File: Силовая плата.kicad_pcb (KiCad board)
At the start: 6 copper layers, 67 x 90.5 mm, 71 parts, among them J1 A, J2 A, J3 B, J4 C, J5 IN-, J6 IN+, J7 Conn_02x10_Odd_Even, J8 A, Q1 2N7002, Q2 2N7002, Q3 2N7002, Q4 2N7002, Q5 2N7002, Q6 2N7002, Q7 BSS214NW

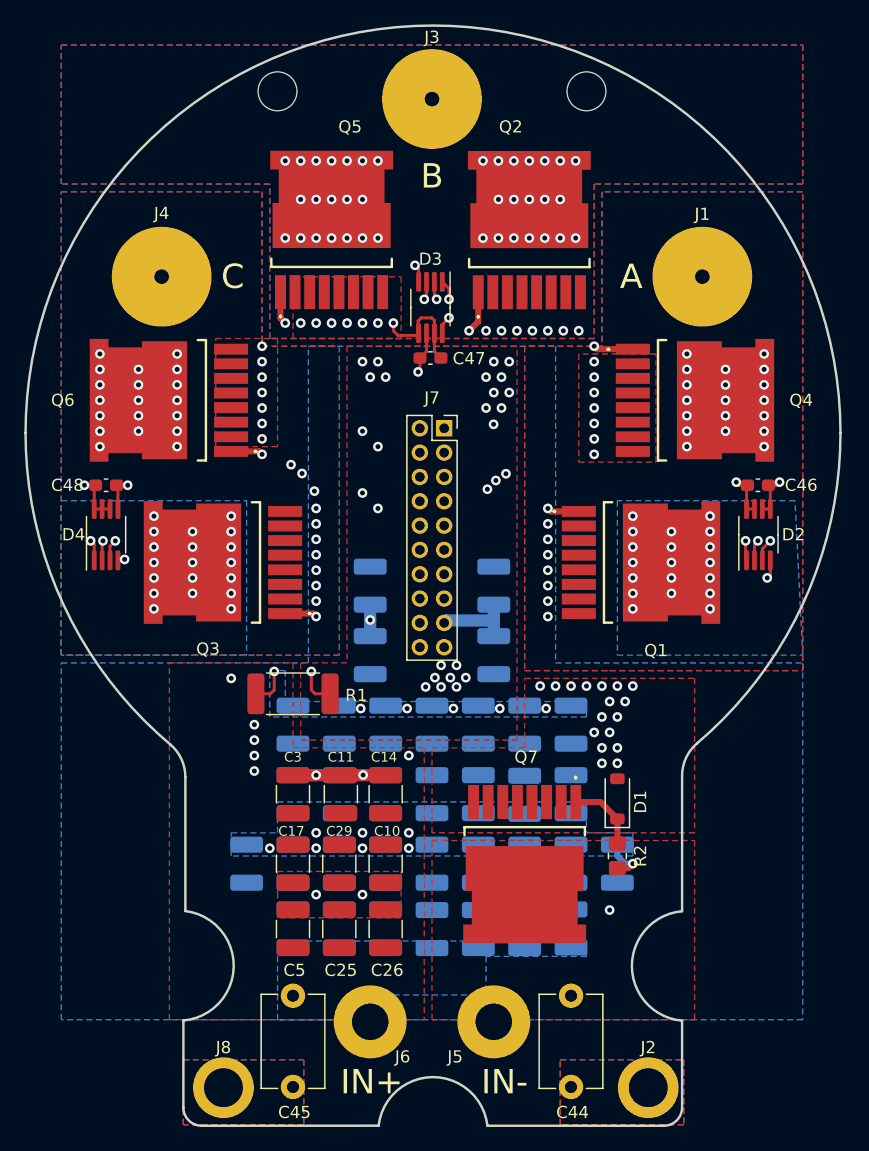
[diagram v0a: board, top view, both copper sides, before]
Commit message: Первый вариант
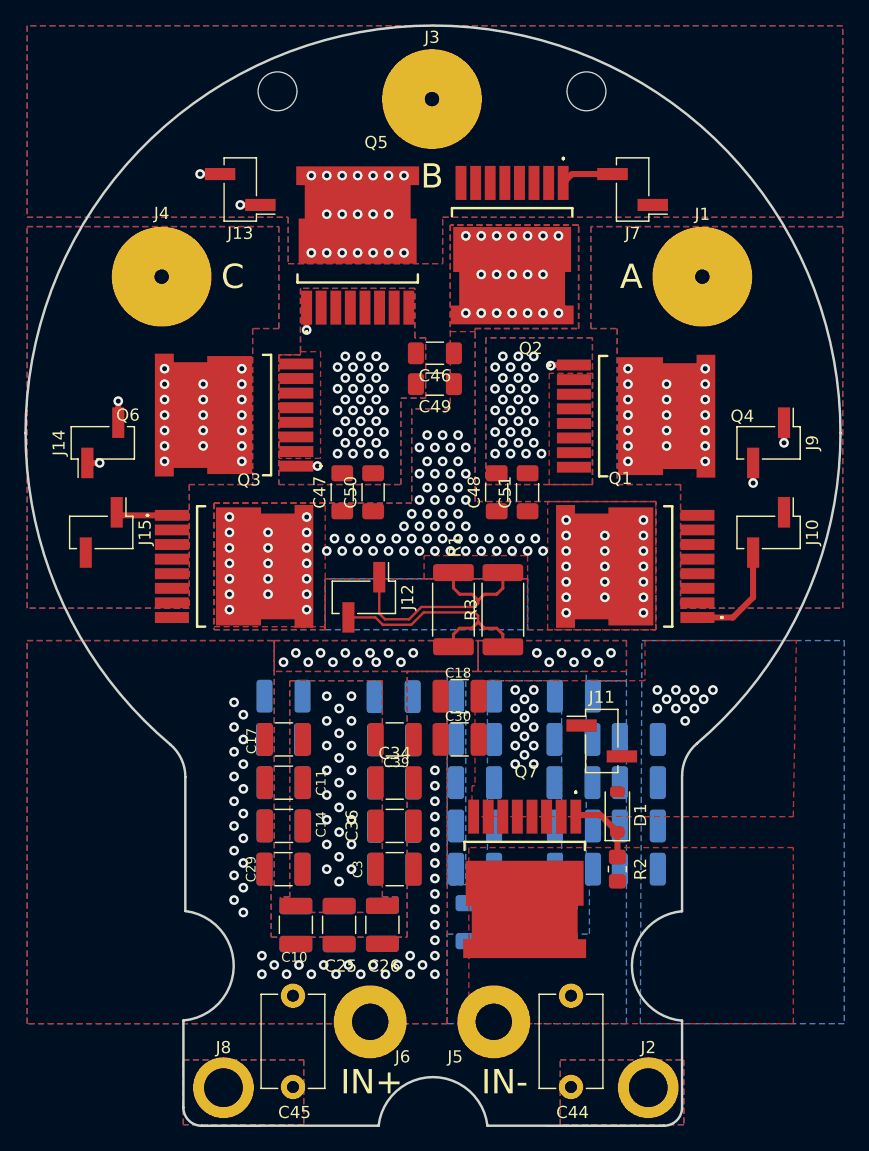
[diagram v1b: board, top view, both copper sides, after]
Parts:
- removed D2, D3, D4: STLM75DS2F, Package_SO:MSOP-8_3x3mm_P0.65mm
- added C49: 10u, Capacitor_SMD:C_1206_3216Metric_Pad1.33x1.80mm_HandSolder, F.Cu at (149.6, 67.1)
- added C50: 10u, Capacitor_SMD:C_1206_3216Metric_Pad1.33x1.80mm_HandSolder, F.Cu at (144.5, 75.9)
- added C51: 10u, Capacitor_SMD:C_1206_3216Metric_Pad1.33x1.80mm_HandSolder, F.Cu at (157.2, 75.9)
- added J10: Conn_01x02_Pin, Connector_PinHeader_2.54mm:PinHeader_1x02_P2.54mm_Vertical_SMD_Pin1Left, F.Cu at (177.0, 79.2)
- added J11: Conn_01x02_Pin, Connector_PinHeader_2.54mm:PinHeader_1x02_P2.54mm_Vertical_SMD_Pin1Left, F.Cu at (163.3, 96.4)
- added J12: Conn_01x02_Pin, Connector_PinHeader_2.54mm:PinHeader_1x02_P2.54mm_Vertical_SMD_Pin1Left, F.Cu at (143.8, 84.6)
- added J13: Conn_01x02_Pin, Connector_PinHeader_2.54mm:PinHeader_1x02_P2.54mm_Vertical_SMD_Pin1Left, F.Cu at (133.6, 51.1)
- added J14: Conn_01x02_Pin, Connector_PinHeader_2.54mm:PinHeader_1x02_P2.54mm_Vertical_SMD_Pin1Left, F.Cu at (122.3, 71.9)
- added J15: Conn_01x02_Pin, Connector_PinHeader_2.54mm:PinHeader_1x02_P2.54mm_Vertical_SMD_Pin1Left, F.Cu at (122.2, 79.2)
- added J9: Conn_01x02_Pin, Connector_PinHeader_2.54mm:PinHeader_1x02_P2.54mm_Vertical_SMD_Pin1Left, F.Cu at (177.0, 71.9)
- added R3: PU2512FKGP60U5L, Resistor_SMD:R_2512_6332Metric_Pad1.40x3.35mm_HandSolder, F.Cu at (155.2, 85.6)
- C18, C30, C34, C36, C39: moved to F.Cu
- C46, C47, C48: value 0.1u -> 10u; footprint Capacitor_SMD:C_0603_1608Metric_Pad1.08x0.95mm_HandSolder -> Capacitor_SMD:C_1206_3216Metric_Pad1.33x1.80mm_HandSolder
- C5: moved to B.Cu
- J7: value Conn_02x10_Odd_Even -> Conn_01x02_Pin; footprint Connector_PinSocket_2.00mm:PinSocket_2x10_P2.00mm_Vertical -> Connector_PinHeader_2.54mm:PinHeader_1x02_P2.54mm_Vertical_SMD_Pin1Left
- moved C12 32.4 mm to (166.4, 103.4), turned to 0 degrees
- moved C48 32.1 mm to (154.7, 75.9), turned to 90 degrees
- moved C5 30.0 mm to (161.0, 92.7), turned to 180 degrees
- moved C22 28.8 mm to (166.4, 99.8), turned to 0 degrees
- moved C46 28.7 mm to (149.6, 64.5), turned to 180 degrees
- moved C24 28.4 mm to (166.4, 106.9), turned to 0 degrees
- moved C32 27.4 mm to (137.2, 92.7), turned to 0 degrees
- moved J7 25.0 mm to (165.9, 51.1), turned to 180 degrees
- moved C28 24.5 mm to (160.0, 111.3)
- moved C23 24.1 mm to (137.1, 96.3), turned to 0 degrees
- moved C36 21.4 mm to (146.3, 103.4), turned to 180 degrees
- moved C39 21.0 mm to (146.3, 96.3), turned to 180 degrees
- moved C40 20.5 mm to (152.9, 92.7), turned to 0 degrees
- moved C16 20.3 mm to (161.0, 106.9), turned to 180 degrees
- moved C38 19.9 mm to (146.3, 103.4), turned to 180 degrees
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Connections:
- C1 pad 1: Shunt_1 -> Shunt+
- C10 pad 1: Shunt_1 -> Shunt+
- C11 pad 1: Shunt_1 -> Shunt+
- C12 pad 1: Shunt_1 -> Shunt+
- C13 pad 1: Shunt_1 -> Shunt+
- C14 pad 1: Shunt_1 -> Shunt+
- C15 pad 1: Shunt_1 -> Shunt+
- C16 pad 1: Shunt_1 -> Shunt+
- C17 pad 1: Shunt_1 -> Shunt+
- C18 pad 1: Shunt_1 -> Shunt+
- C19 pad 1: Shunt_1 -> Shunt+
- C2 pad 1: Shunt_1 -> Shunt+
- C20 pad 1: Shunt_1 -> Shunt+
- C21 pad 1: Shunt_1 -> Shunt+
- C22 pad 1: Shunt_1 -> Shunt+
- C23 pad 1: Shunt_1 -> Shunt+
- C24 pad 1: Shunt_1 -> Shunt+
- C25 pad 1: Shunt_1 -> Shunt+
- C26 pad 1: Shunt_1 -> Shunt+
- C27 pad 1: Shunt_1 -> Shunt+
- C28 pad 1: Shunt_1 -> Shunt+
- C29 pad 1: Shunt_1 -> Shunt+
- C3 pad 1: Shunt_1 -> Shunt+
- C30 pad 1: Shunt_1 -> Shunt+
- C31 pad 1: Shunt_1 -> Shunt+
- C32 pad 1: Shunt_1 -> Shunt+
- C33 pad 1: Shunt_1 -> Shunt+
- C34 pad 1: Shunt_1 -> Shunt+
- C35 pad 1: Shunt_1 -> Shunt+
- C36 pad 1: Shunt_1 -> Shunt+
- C37 pad 1: Shunt_1 -> Shunt+
- C38 pad 1: Shunt_1 -> Shunt+
- C39 pad 1: Shunt_1 -> Shunt+
- C4 pad 1: Shunt_1 -> Shunt+
- C40 pad 1: Shunt_1 -> Shunt+
- C41 pad 1: Shunt_1 -> Shunt+
- C42 pad 1: Shunt_1 -> Shunt+
- C43 pad 1: Shunt_1 -> Shunt+
- C45 pad 1: Shunt_1 -> Shunt+
- C46 pad 1: +3.3V -> Shunt-
- C47 pad 1: +3.3V -> Shunt-
- C48 pad 1: +3.3V -> Shunt-
- C5 pad 1: Shunt_1 -> Shunt+
- C6 pad 1: Shunt_1 -> Shunt+
- C7 pad 1: Shunt_1 -> Shunt+
- C8 pad 1: Shunt_1 -> Shunt+
- C9 pad 1: Shunt_1 -> Shunt+
- J6 pad 1: Shunt_1 -> Shunt+
- J7 pad 1: +3.3V -> B
- J7 pad 2: ~{OS}_MCU -> G3
- Q1 pad 3: Shunt_2 -> Shunt-
- Q2 pad 3: Shunt_2 -> Shunt-
- Q3 pad 3: Shunt_2 -> Shunt-
- R1 pad 1: Shunt_1 -> Shunt+
- R1 pad 2: Shunt_2 -> Shunt-
- R2 pad 2: Shunt_1 -> Shunt+
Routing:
- net +3.3V: track 100.2 -> 0.00 mm, vias 4 -> 0
- net SDA_MCU: track 84.2 -> 0.00 mm, vias 5 -> 0
- net ~{OS}_MCU: track 82.2 -> 0.00 mm, vias 5 -> 0
- net SCL_MCU: track 79.1 -> 0.00 mm, vias 5 -> 0
- net Shunt_1: track 63.3 -> 0.00 mm, vias 21 -> 0
- net GND: track 28.5 -> 5.08 mm, vias 48 -> 118
- net Shunt-: track 0.00 -> 19.6 mm, vias 0 -> 116
- net Shunt+: track 0.00 -> 18.9 mm, vias 0 -> 67
- net B: track 13.4 -> 0.00 mm, vias 26 -> 19
- net Shunt_2: track 12.8 -> 0.00 mm, vias 83 -> 0
- net A: track 10.2 -> 0.00 mm, vias 26 -> 19
- net G3: track 14.6 -> 4.35 mm, vias 1 -> 0
- net C: track 9.44 -> 0.00 mm, vias 26 -> 19
- net G2: track 21.1 -> 28.4 mm, vias 1 -> 2
- net G5: track 11.8 -> 4.64 mm, vias 1 -> 0
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- added copper zone on In3.Cu, net A
- added copper zone on In3.Cu, net B
- added copper zone on In3.Cu, net C
- added copper zone on In3.Cu, net GND
- added copper zone on B.Cu, net Shunt+
- added copper zone on F.Cu, net Shunt+
- added copper zone on In2.Cu, net Shunt+
- added copper zone on In4.Cu, net Shunt+
- added copper zone on B.Cu, net Shunt-
- added copper zone on F.Cu, net Shunt-
- added copper zone on In2.Cu, net Shunt-
- added copper zone on In3.Cu, net Shunt-
- added copper zone on In4.Cu, net Shunt-
- removed copper zone on B.Cu, net Shunt_1
- removed copper zone on F.Cu, net Shunt_1
- removed copper zone on In3.Cu, net Shunt_1
- removed copper zone on B.Cu, net Shunt_2
- removed copper zone on F.Cu, net Shunt_2
- removed copper zone on In3.Cu, net Shunt_2
